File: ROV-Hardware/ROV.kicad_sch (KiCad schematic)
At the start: 28 parts, among them J1 T-block, J2 T-block, J3 Screw_Terminal_01x04, SW1 switch, U1 LM7812, U2 LM7805, U3 ESP32-S3-DEVKITC-1-N8R2, U4 MPU6050, U5 ZK-BM1, U6 ZK-BM1, U7 ZK-BM1, U8 A4988, U9 GY-MS5837

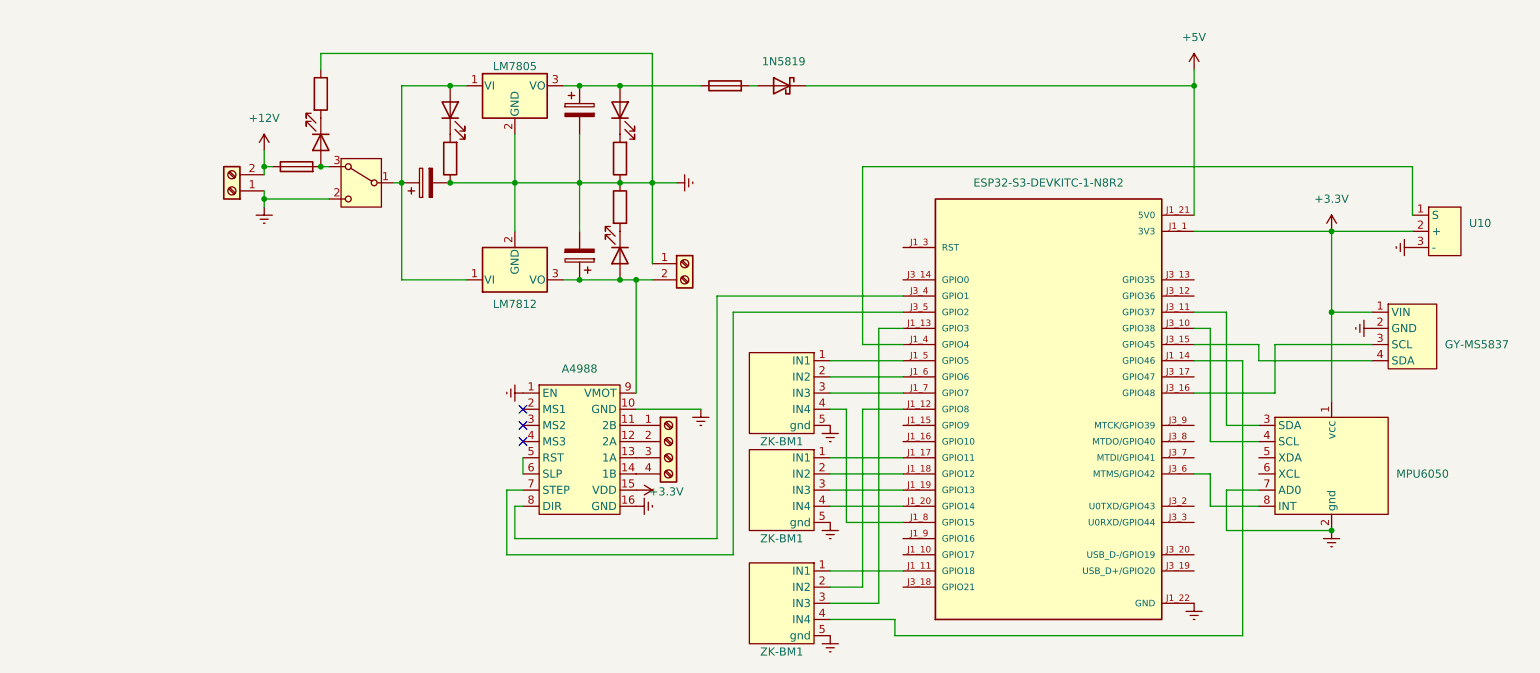
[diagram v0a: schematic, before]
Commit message: hight current
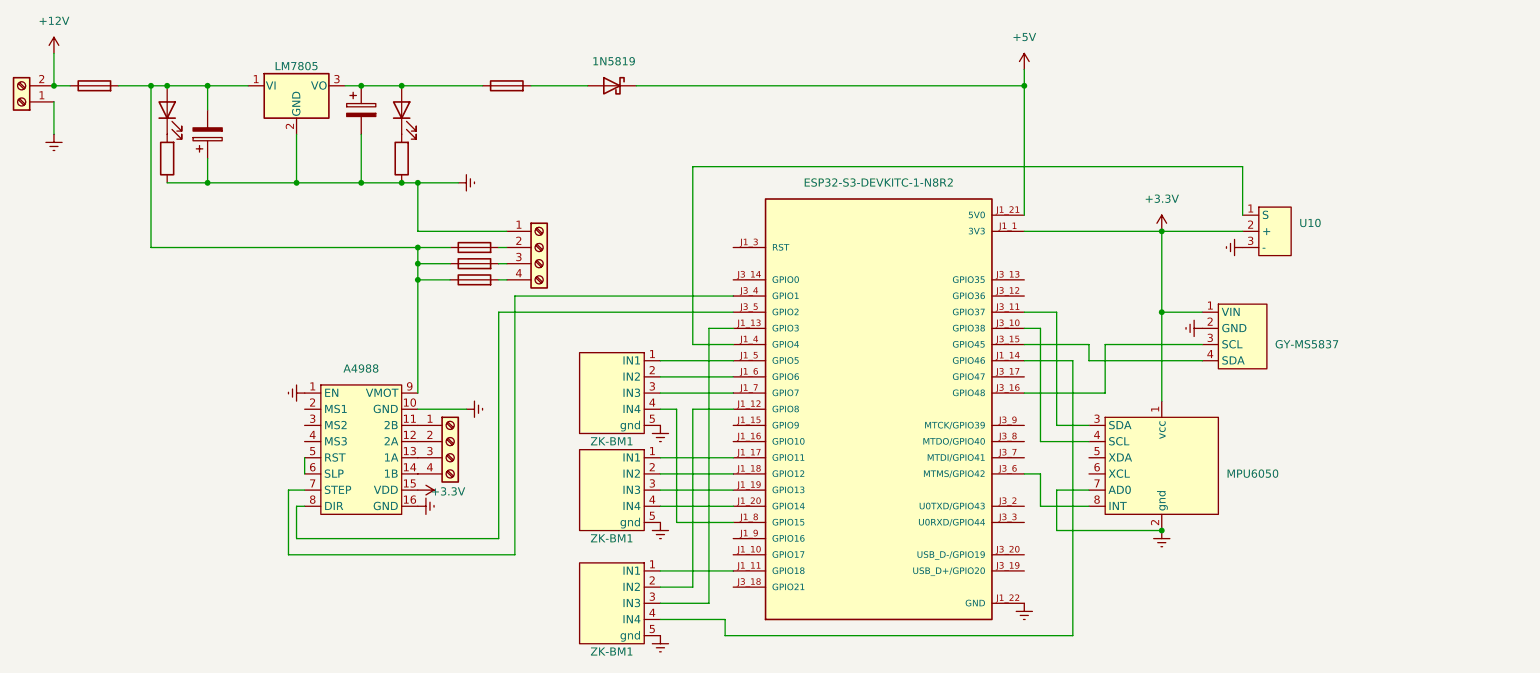
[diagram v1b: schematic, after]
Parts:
- removed C3: capacitor, Capacitor_THT:CP_Radial_D5.0mm_P2.50mm, symbol Device:C_Polarized
- removed D4, D5: LED, LED_THT:LED_D3.0mm, symbol Device:LED
- removed J2: T-block, TerminalBlock:TerminalBlock_MaiXu_MX126-5.0-02P_1x02_P5.00mm, symbol Connector:Screw_Terminal_01x02
- removed R3, R4: R, Resistor_THT:R_Axial_DIN0204_L3.6mm_D1.6mm_P5.08mm_Horizontal, symbol Device:R
- removed SW1: switch, Button_Switch_THT:SW_Slide-03_Wuerth-WS-SLTV_10x2.5x6.4_P2.54mm, symbol Switch:SW_Wuerth_450301014042
- removed U1: LM7812, Package_TO_SOT_THT:TO-220-3_Vertical, symbol Regulator_Linear:LM7812_TO220
- added F3, F4, F5: fuse, Fuse:Fuseholder_Clip-5x20mm_Schurter_CQM_Inline_P20.60x5.00mm_D1.00mm_Horizontal, symbol Device:Fuse
- added J2: Screw_Terminal_01x04, TerminalBlock:TerminalBlock_MaiXu_MX126-5.0-04P_1x04_P5.00mm, symbol Connector:Screw_Terminal_01x04
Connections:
- net GND: now also C1.1, J2.1 (Pin_1); no longer C1.2
- net at U3.J3_4 (GPIO1): now also U8.7 (STEP); no longer U8.8 (DIR)
- net at U3.J3_5 (GPIO2): now also U8.8 (DIR); no longer U8.7 (STEP)
- net at U8.9 (VMOT): now also C1.2, D2.2 (A), F1.2, U2.1 (VI), F3.1, F4.1, F5.1
- new net: F5.2, J2.4 (Pin_4)
- new net: F4.2, J2.3 (Pin_3)
- new net: F3.2, J2.2 (Pin_2)
- no-connect marks 3 -> 0
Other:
- moved on the sheet: U10
